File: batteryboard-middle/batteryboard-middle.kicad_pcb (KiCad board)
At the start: 2 copper layers, 46.8 x 46.8 mm, 9 parts, among them J1 FLE-105-01-G-DV-A, J2 Conn_01x02, J3 Conn_01x02, J4 FTS-105-01-L-DV-A

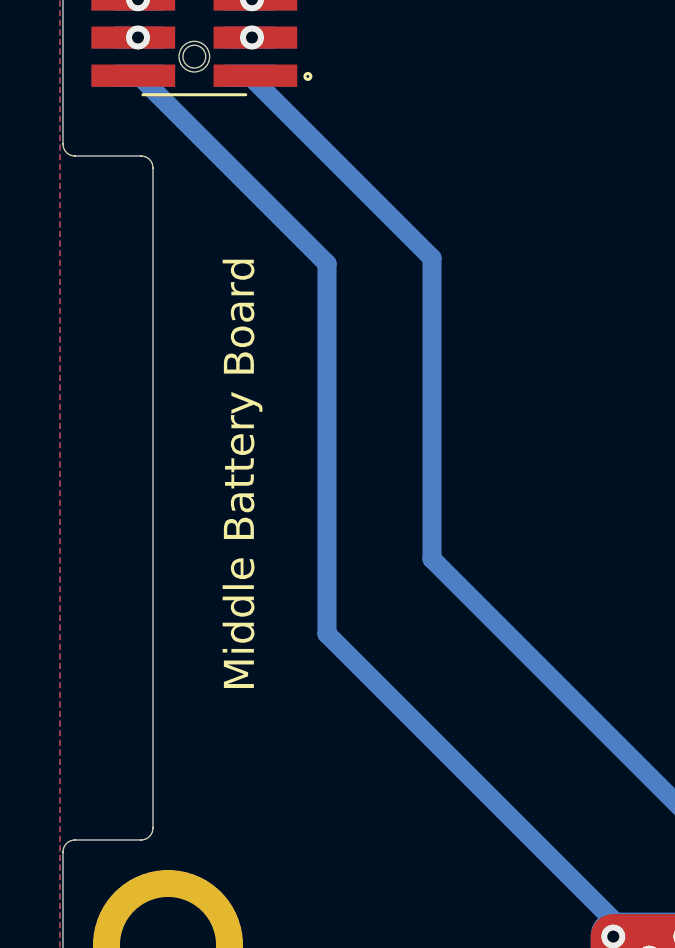
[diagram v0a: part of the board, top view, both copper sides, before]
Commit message: Export New Gerbers
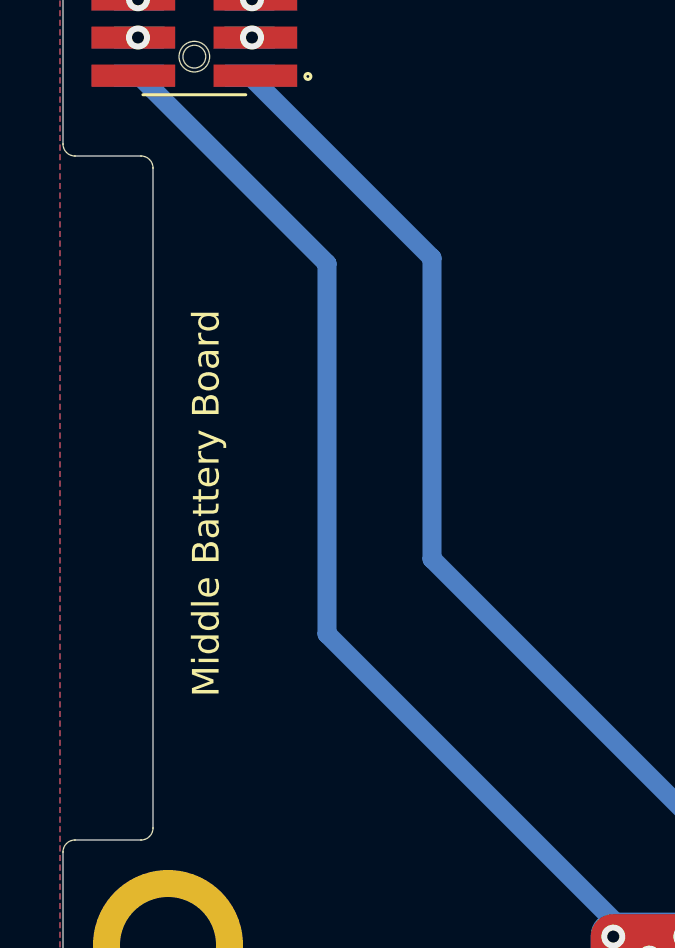
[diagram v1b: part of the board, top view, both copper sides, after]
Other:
- board text added: "06-JUL-22"
- board text added: "v01.1"
- board text removed: "09-JUN-22"
- board text removed: "v01"
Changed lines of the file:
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@@
       (outputformat 1)
       (mirror false)
-      (drillshape 1)
+      (drillshape 0)
       (scaleselection 1)
-      (outputdirectory "")
+      (outputdirectory "../gerbers/batteryboard-middle (07-06-22)/")
     )
   )
@@
     (effects (font (size 4 4) (thickness 0.7)) (justify mirror))
   )
-  (gr_text "Middle Battery Board\n" (at 129.3 104.8 90) (layer "F.SilkS")
-    (effects (font (size 1 1) (thickness 0.15)))
+  (gr_text "Middle Battery Board\n" (at 128.175 105.775 90) (layer "F.SilkS")
+    (effects (font (size 0.889 0.889) (thickness 0.127)))
   )
   (gr_text "-" (at 137.8 120.6) (layer "F.SilkS")
     (effects (font (size 4 4) (thickness 0.7)) (justify mirror))
   )
-  (gr_text "09-JUN-22" (at 148.7 79.9) (layer "F.Mask")
+  (gr_text "06-JUL-22" (at 148.7 79.9) (layer "F.Mask")
     (effects (font (size 0.635 0.635) (thickness 0.1524)) (justify right))
   )
-  (gr_text "v01" (at 150.681203 82.287588) (layer "F.Mask")
+  (gr_text "v01.1" (at 150.681203 82.287588) (layer "F.Mask")
     (effects (font (size 0.635 0.635) (thickness 0.1524)) (justify right))
   )
